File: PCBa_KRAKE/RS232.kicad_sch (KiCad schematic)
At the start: 19 parts

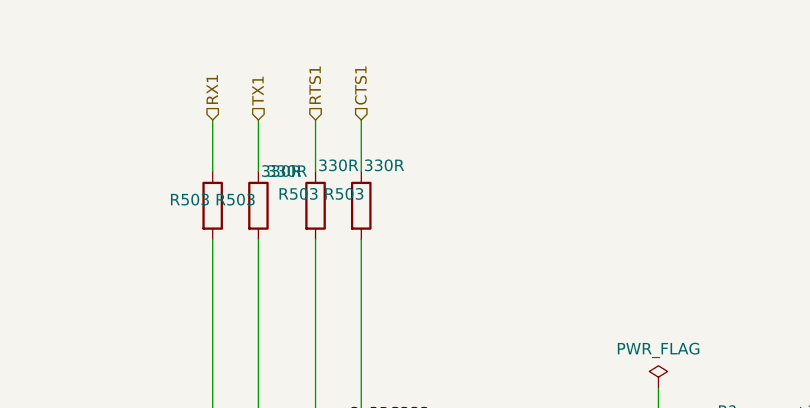
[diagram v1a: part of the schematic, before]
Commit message: PLacing and routing, Added new EMC resistors at the output of the microcoontroller.
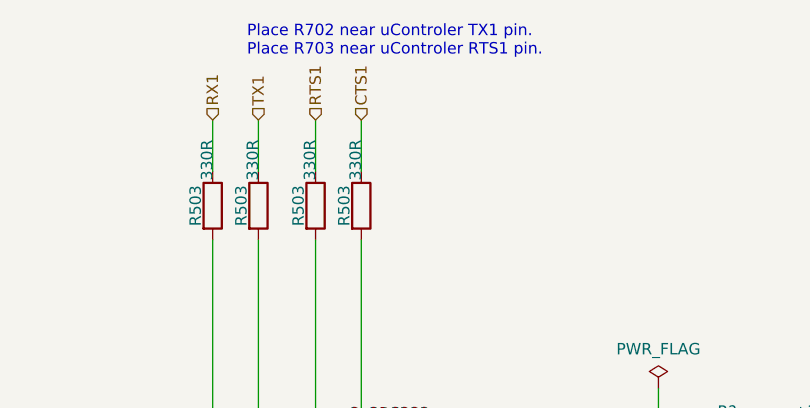
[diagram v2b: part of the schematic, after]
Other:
- note added: "Place R702 near uControler TX1 pin. Place R703 near uControler RTS1 pin."
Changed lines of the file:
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@@
     (stroke (width 0) (type default))
+  )
+  (text "Place R702 near uControler TX1 pin.\nPlace R703 near uControler RTS1 pin."
+    (at 130.81 30.48 0)
+    (effects (font (size 1.27 1.27)) (justify left bottom))
   )
   (text "NULL MODEM" (at 159.385 114.3 0)
@@
   (symbol (lib_id "Device:R") (at 132.08 46.99 0) (unit 1)
     (in_bom yes) (on_board yes) (dnp no)
-    (property "Reference" "R503" (at 129.54 46.355 0)
-      (effects (font (size 1.27 1.27)))
-    )
-    (property "Value" "330R" (at 134.62 43.18 0)
+    (property "Reference" "R503" (at 130.175 46.99 90)
+      (effects (font (size 1.27 1.27)))
+    )
+    (property "Value" "330R" (at 131.445 41.91 90)
       (effects (font (size 1.27 1.27)))
     )
@@
   (symbol (lib_id "Device:R") (at 138.43 46.99 0) (unit 1)
     (in_bom yes) (on_board yes) (dnp no)
-    (property "Reference" "R503" (at 136.525 45.72 0)
-      (effects (font (size 1.27 1.27)))
-    )
-    (property "Value" "330R" (at 140.97 42.545 0)
+    (property "Reference" "R503" (at 136.525 46.99 90)
+      (effects (font (size 1.27 1.27)))
+    )
+    (property "Value" "330R" (at 137.795 41.91 90)
       (effects (font (size 1.27 1.27)))
     )
@@
   (symbol (lib_id "Device:R") (at 143.51 46.99 0) (unit 1)
     (in_bom yes) (on_board yes) (dnp no)
-    (property "Reference" "R503" (at 141.605 45.72 0)
-      (effects (font (size 1.27 1.27)))
-    )
-    (property "Value" "330R" (at 146.05 42.545 0)
+    (property "Reference" "R503" (at 141.605 46.99 90)
+      (effects (font (size 1.27 1.27)))
+    )
+    (property "Value" "330R" (at 142.875 41.91 90)
       (effects (font (size 1.27 1.27)))
     )
@@
   (symbol (lib_id "Device:R") (at 127 46.99 0) (unit 1)
     (in_bom yes) (on_board yes) (dnp no)
-    (property "Reference" "R503" (at 124.46 46.355 0)
-      (effects (font (size 1.27 1.27)))
-    )
-    (property "Value" "330R" (at 135.255 43.18 0)
-      (effects (font (size 1.27 1.27)))
-    )
+    (property "Reference" "R503" (at 125.095 46.99 90)
+      (effects (font (size 1.27 1.27)))
+    )
+    (property "Value" "330R" (at 126.365 41.91 90)
+      (effects (font (size 1.27 1.27)))
+    )

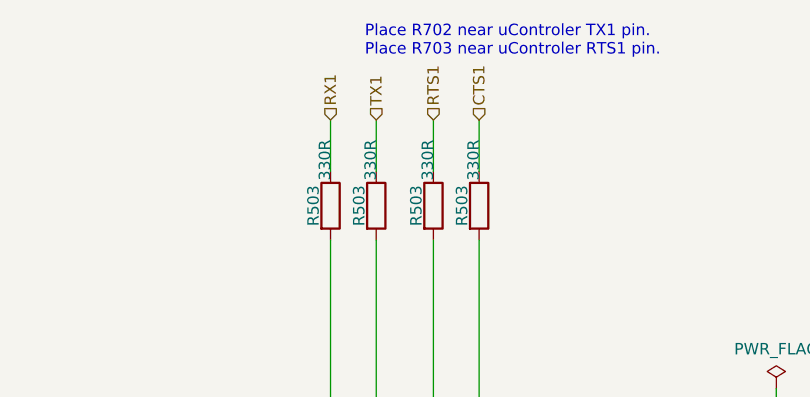
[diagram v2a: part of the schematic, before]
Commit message: Corrected the voltage connection for the mute switch, from 5V to 3V3. Rerouted and reconnected the tracks for R603.
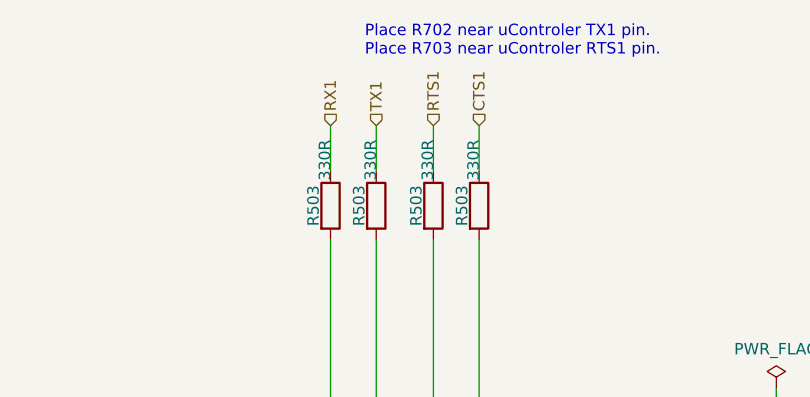
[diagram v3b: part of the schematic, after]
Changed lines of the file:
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@@
   (no_connect (at 187.96 134.62))
   (no_connect (at 187.96 116.84))
-  (wire (pts (xy 127 37.465) (xy 127 43.18))
+  (wire (pts (xy 127 38.1) (xy 127 43.18))
     (stroke (width 0) (type default))
   )
@@
     (stroke (width 0) (type default))
   )
-  (wire (pts (xy 138.43 37.465) (xy 138.43 43.18))
+  (wire (pts (xy 138.43 38.1) (xy 138.43 43.18))
     (stroke (width 0) (type default))
   )
@@
     (stroke (width 0) (type default))
   )
-  (wire (pts (xy 132.08 37.465) (xy 132.08 43.18))
+  (wire (pts (xy 132.08 38.1) (xy 132.08 43.18))
     (stroke (width 0) (type default))
   )
@@
     (stroke (width 0) (type default))
   )
-  (wire (pts (xy 143.51 37.465) (xy 143.51 43.18))
+  (wire (pts (xy 143.51 38.1) (xy 143.51 43.18))
     (stroke (width 0) (type default))
   )
@@
     (effects (font (size 1.27 1.27)) (justify left bottom))
   )
-  (hierarchical_label "CTS1" (shape input) (at 143.51 37.465 90) (fields_autoplaced)
-    (effects (font (size 1.27 1.27)) (justify left))
-  )
-  (hierarchical_label "TX1" (shape input) (at 132.08 37.465 90) (fields_autoplaced)
-    (effects (font (size 1.27 1.27)) (justify left))
-  )
-  (hierarchical_label "RX1" (shape input) (at 127 37.465 90) (fields_autoplaced)
-    (effects (font (size 1.27 1.27)) (justify left))
-  )
-  (hierarchical_label "RTS1" (shape input) (at 138.43 37.465 90) (fields_autoplaced)
-    (effects (font (size 1.27 1.27)) (justify left))
-  )
+  (hierarchical_label "CTS1" (shape input) (at 143.51 38.1 90) (fields_autoplaced)
+    (effects (font (size 1.27 1.27)) (justify left))
+  )
+  (hierarchical_label "TX1" (shape input) (at 132.08 38.1 90) (fields_autoplaced)
+    (effects (font (size 1.27 1.27)) (justify left))
+  )
+  (hierarchical_label "RX1" (shape input) (at 127 38.1 90) (fields_autoplaced)
+    (effects (font (size 1.27 1.27)) (justify left))
+  )
+  (hierarchical_label "RTS1" (shape input) (at 138.43 38.1 90) (fields_autoplaced)
+    (effects (font (size 1.27 1.27)) (justify left))
+  )

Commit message: Found missing part numbers. ESP32.
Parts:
- U?: Distributor 1 (none) -> JLCPCB
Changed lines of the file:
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@@
+      (effects (font (size 1.27 1.27)) hide)
+    )
+    (property "Distributor 1" "JLCPCB" (at 104.14 106.68 0)
       (effects (font (size 1.27 1.27)) hide)
     )
